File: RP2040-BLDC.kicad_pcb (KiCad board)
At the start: 4 copper layers, 40.2 x 35.8 mm, 33 parts, among them J1 Motor, J2 Conn_01x02, J3 USB_B_Micro, J4 Motor power, U2 AS5048A, U6 RP2040

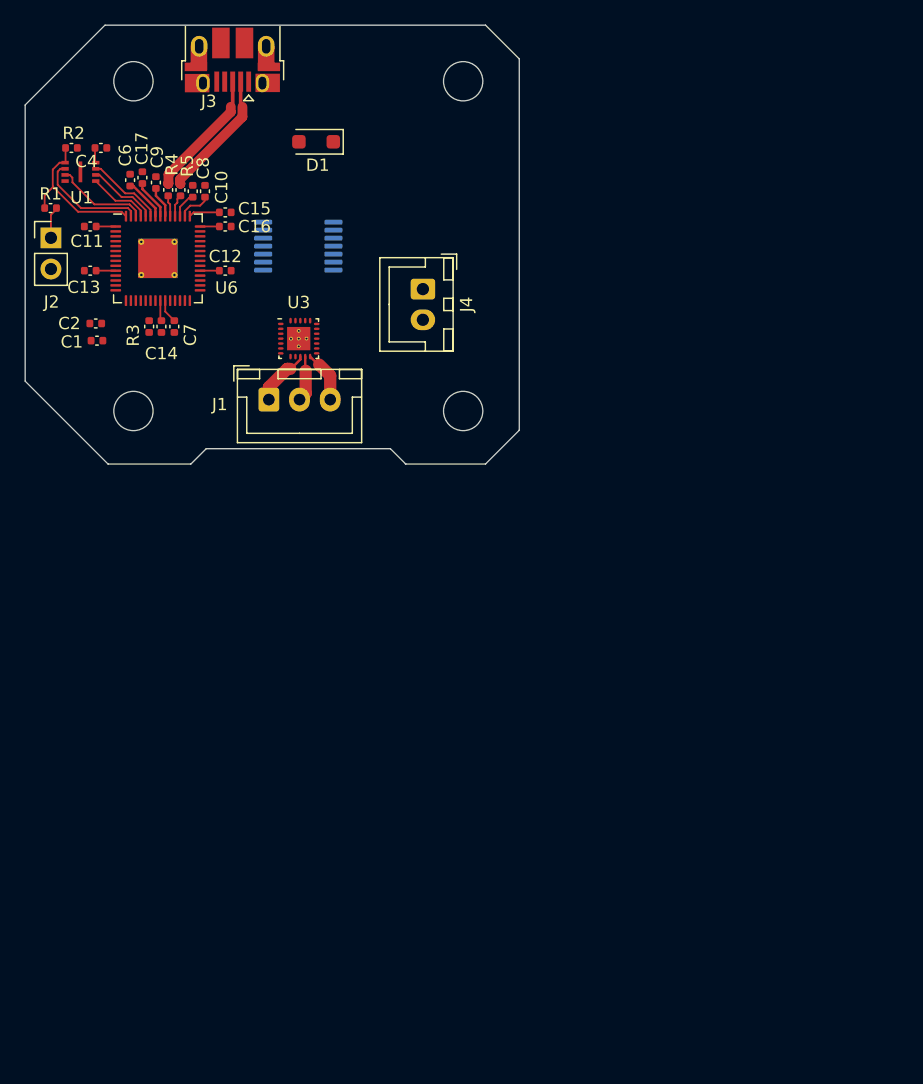
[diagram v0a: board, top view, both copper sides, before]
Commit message: WIP
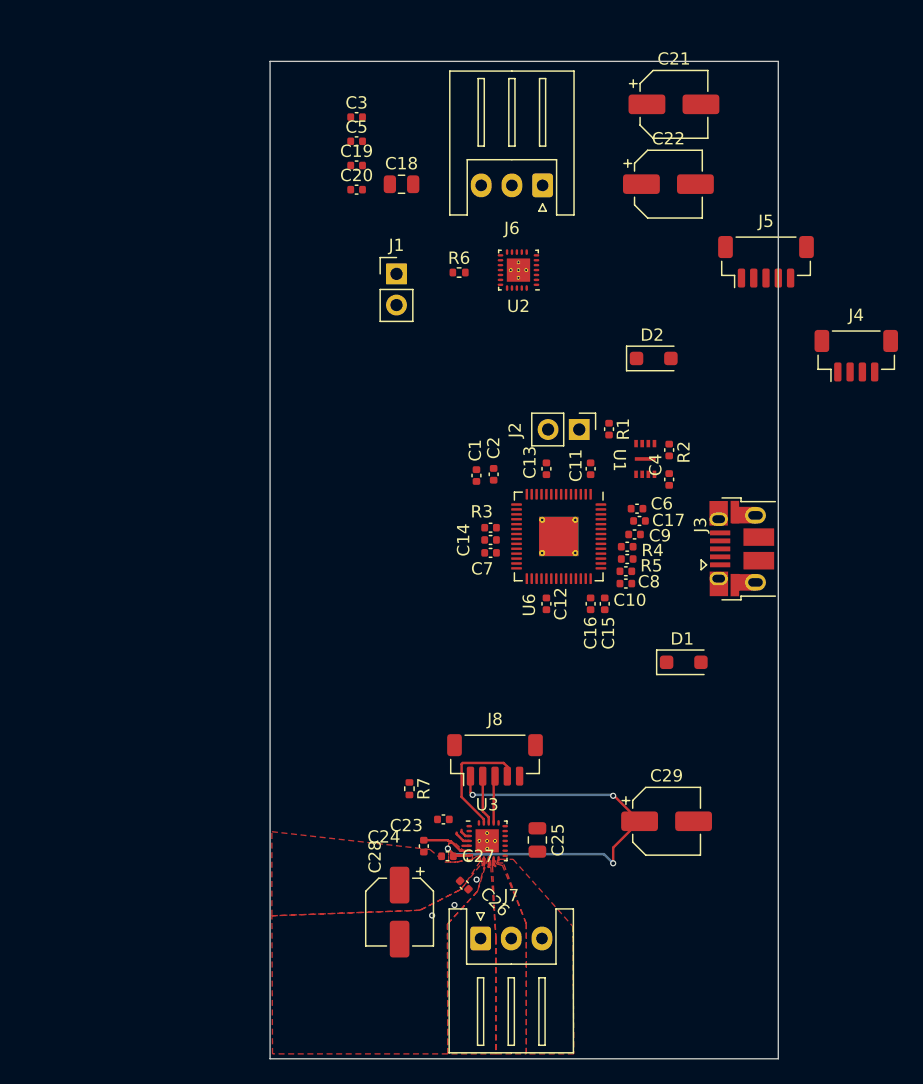
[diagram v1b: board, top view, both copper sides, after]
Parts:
- removed H1, H2, H3, H4: MountingHole, MountingHole:MountingHole_3.2mm_M3
- added C18: 4.7u, Capacitor_SMD:C_0805_2012Metric, F.Cu at (58.4, 45.0)
- added C19: 0.1u, Capacitor_SMD:C_0402_1005Metric, F.Cu at (54.8, 43.4)
- added C20: 0.1u, Capacitor_SMD:C_0402_1005Metric, F.Cu at (54.8, 45.4)
- added C21: 22u, Capacitor_SMD:CP_Elec_5x5.4, F.Cu at (80.6, 38.5)
- added C22: 22u, Capacitor_SMD:CP_Elec_5x5.4, F.Cu at (80.2, 45.0)
- added C23: 0.1u, Capacitor_SMD:C_0402_1005Metric, F.Cu at (61.8, 96.7)
- added C24: 0.1u, Capacitor_SMD:C_0402_1005Metric, F.Cu at (60.2, 98.9)
- added C25: 4.7u, Capacitor_SMD:C_0805_2012Metric, F.Cu at (69.5, 98.4)
- added C26: 0.1u, Capacitor_SMD:C_0402_1005Metric, F.Cu at (63.5, 102.0)
- added C27: 0.1u, Capacitor_SMD:C_0402_1005Metric, F.Cu at (62.1, 99.7)
- added C28: 22u, Capacitor_SMD:CP_Elec_5x5.4, F.Cu at (58.2, 104.2)
- added C29: 22u, Capacitor_SMD:CP_Elec_5x5.4, F.Cu at (80.0, 96.8)
- added C3: 0.1u, Capacitor_SMD:C_0402_1005Metric, F.Cu at (54.8, 39.5)
- added C5: 0.1u, Capacitor_SMD:C_0402_1005Metric, F.Cu at (54.8, 41.5)
- added D2: MBR1020VL, Diode_SMD:D_SOD-123F, F.Cu at (79.0, 59.1)
- added J5: AS5048A, Connector_JST:JST_SH_BM05B-SRSS-TB_1x05-1MP_P1.00mm_Vertical, F.Cu at (88.1, 51.3)
- added J6: M1, Connector_JST:JST_XH_S3B-XH-A_1x03_P2.50mm_Horizontal, F.Cu at (69.9, 45.0)
- added J7: M2, Connector_JST:JST_XH_S3B-XH-A_1x03_P2.50mm_Horizontal, F.Cu at (64.8, 106.4)
- added J8: AS5048A, Connector_JST:JST_SH_BM05B-SRSS-TB_1x05-1MP_P1.00mm_Vertical, F.Cu at (66.0, 91.8)
- added R6: 5.1k, Resistor_SMD:R_0402_1005Metric, F.Cu at (63.1, 52.1)
- added R7: 5.1k, Resistor_SMD:R_0402_1005Metric, F.Cu at (59.0, 94.2)
- J1: value Motor -> MPWR; footprint Connector_JST:JST_XH_B3B-XH-A_1x03_P2.50mm_Vertical -> Connector_PinHeader_2.54mm:PinHeader_1x02_P2.54mm_Vertical
- J4: value Motor power -> I2C5V; footprint Connector_JST:JST_XH_B2B-XH-A_1x02_P2.50mm_Vertical -> Connector_JST:JST_SH_BM04B-SRSS-TB_1x04-1MP_P1.00mm_Vertical
- U2: value AS5048A -> ~; footprint Package_SO:TSSOP-14_4.4x5mm_P0.65mm -> MyLibrary:WQFN-24_EP_2.93x2.93_Pitch0.4mm; moved to F.Cu
- moved J3 57.5 mm to (86.1, 74.6), turned to 90 degrees
- moved R2 54.6 mm to (80.2, 66.6), turned to 90 degrees
- moved C4 53.6 mm to (80.2, 69.0), turned to -90 degrees
- moved D1 51.9 mm to (81.4, 83.9), turned to 0 degrees
- moved U1 50.3 mm to (77.3, 67.3), turned to -90 degrees
- moved C17 49.2 mm to (77.8, 72.4), turned to 0 degrees
- moved C6 49.2 mm to (77.6, 71.4), turned to 0 degrees
- moved R1 48.9 mm to (75.3, 64.9), turned to -90 degrees
- moved C9 48.4 mm to (77.4, 73.5), turned to 0 degrees
- moved R4 47.4 mm to (76.8, 74.5), turned to 180 degrees
- moved R5 47.2 mm to (76.8, 75.5), turned to 180 degrees
- moved C8 46.9 mm to (76.7, 76.5), turned to 0 degrees
- moved C10 46.9 mm to (76.7, 77.5), turned to 0 degrees
- moved J2 45.8 mm to (72.9, 64.9), turned to -90 degrees
- moved C11 45.3 mm to (73.8, 68.1), turned to 90 degrees
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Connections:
- D1 pad 1: VCOM -> +5V
- J1 pad 1: /M1 -> GND
- J1 pad 2: /M2 -> +BATT
- J4 pad 1: GND -> /I2C0_SCL
- J4 pad 2: Vdrive -> /I2C0_SDA
- U2 pad 1: unconnected-(U2-~{CSn}-Pad1) -> /Driver sensor pair/DRV~{FAULT}
- U2 pad 10: unconnected-(U2-TEST-Pad10) -> /Driver sensor pair/MA
- U2 pad 11: unconnected-(U2-VDD5V-Pad11) -> /Driver sensor pair/MB
- U2 pad 12: unconnected-(U2-VDD3V-Pad12) -> /Driver sensor pair/MC
- U2 pad 2: unconnected-(U2-CLK-Pad2) -> Net-(U2-CSAREF)
- U2 pad 3: unconnected-(U2-MISO-Pad3) -> /Driver sensor pair/SOC
- U2 pad 4: unconnected-(U2-MOSI-Pad4) -> /Driver sensor pair/SOB
- U2 pad 5: unconnected-(U2-TEST-Pad5) -> /Driver sensor pair/SOA
- U2 pad 6: unconnected-(U2-TEST-Pad6) -> Net-(U2-CP)
- U2 pad 7: unconnected-(U2-TEST-Pad7) -> +5V
- U2 pad 8: unconnected-(U2-TEST-Pad8) -> +BATT
- U2 pad 9: unconnected-(U2-TEST-Pad9) -> GND
- U3 pad 1: unconnected-(U3-~{FAULT}-Pad1) -> /Driver sensor pair1/DRV~{FAULT}
- U3 pad 10: /M1 -> /Driver sensor pair1/MA
- U3 pad 11: /M2 -> /Driver sensor pair1/MB
- U3 pad 12: /M3 -> /Driver sensor pair1/MC
- U3 pad 17: unconnected-(U3-AVDD-Pad17) -> /Driver sensor pair1/3.3VOUT
- U3 pad 19: unconnected-(U3-PWM_SYNC-Pad19) -> /Driver sensor pair1/PWM_SYNC
- U3 pad 2: unconnected-(U3-CSAREF-Pad2) -> Net-(U3-CSAREF)
- U3 pad 20: /DRV_CSn -> /Driver sensor pair1/DRV~{CS}
- U3 pad 21: /SPI0_RX -> /Driver sensor pair1/SDO
- U3 pad 22: /SPI0_TX -> /Driver sensor pair1/SDI
- U3 pad 23: /SPI0_SCK -> /Driver sensor pair1/SPI_CLK
- U3 pad 24: unconnected-(U3-~{SLEEP}-Pad24) -> /Driver sensor pair1/~{SLEEP}
- U3 pad 25: (no net) -> GND
- U3 pad 3: unconnected-(U3-SOC-Pad3) -> /Driver sensor pair1/SOC
- U3 pad 4: unconnected-(U3-SOB-Pad4) -> /Driver sensor pair1/SOB
- U3 pad 5: unconnected-(U3-SOA-Pad5) -> /Driver sensor pair1/SOA
- U3 pad 6: unconnected-(U3-CP-Pad6) -> Net-(U3-CP)
- U3 pad 7: VCOM -> +5V
- U3 pad 8: Vdrive -> +BATT
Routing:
- net +5V: track 0.00 -> 36.9 mm, vias 0 -> 4
- net +3V3: track 19.9 -> 0.00 mm
- net /QSPI_SS: track 12.8 -> 0.00 mm
- net /USB_D+: track 10.5 -> 0.00 mm
- net /USB_D-: track 10.5 -> 0.00 mm
- net /Driver sensor pair1/SPI_CLK: track 0.00 -> 10.2 mm
- net /QSPI_SD1: track 9.04 -> 0.00 mm
- net /QSPI_SD2: track 7.64 -> 0.00 mm
- net +1V1: track 7.51 -> 0.00 mm
- net /QSPI_SD3: track 6.37 -> 0.00 mm
- net /QSPI_SCLK: track 5.75 -> 0.00 mm
- net /QSPI_SD0: track 5.13 -> 0.00 mm
- net /M1: track 4.74 -> 0.00 mm
- net /M3: track 4.23 -> 0.00 mm
- net Net-(U3-CP): track 0.00 -> 4.05 mm
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- added copper zone on F.Cu, net +5V
- added copper zone on F.Cu, net +BATT
- added copper zone on F.Cu, net /Driver sensor pair1/MA
- added copper zone on F.Cu, net /Driver sensor pair1/MB
- added copper zone on F.Cu, net /Driver sensor pair1/MC
- added copper zone on F.Cu, net GND
- added copper zone on In1.Cu, net GND
- added copper zone on In2.Cu, net GND
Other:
- board size 40.2 x 35.8 mm -> 41.4 x 81.2 mm
